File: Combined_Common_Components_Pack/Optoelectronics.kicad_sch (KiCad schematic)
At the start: 7 parts, among them U6 PC817XI

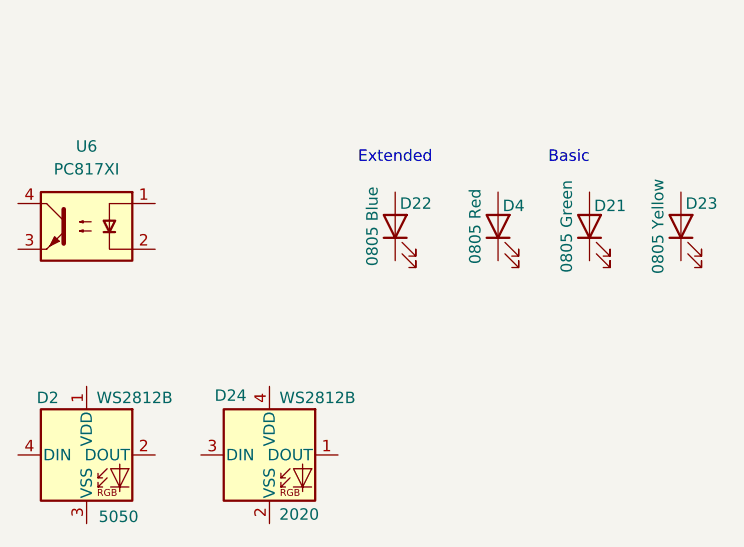
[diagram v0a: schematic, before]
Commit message: More circuits
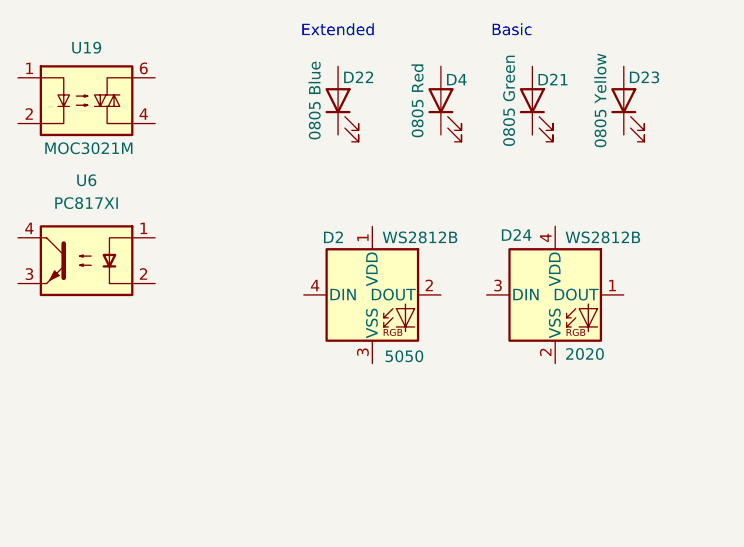
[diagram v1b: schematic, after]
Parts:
- added U19: MOC3021M, Package_DIP:SMDIP-6_W9.53mm, symbol Relay_SolidState:MOC3021M
- U6: Type SMD -> (none)
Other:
- moved on the sheet: D2, D21, D22, D23, D24, D4, U6
